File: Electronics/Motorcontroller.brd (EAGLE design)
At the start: 100 x 48.2 mm, 27 parts, among them Q1 IRFZ48V, Q2 IRF4905V, Q3 IRFZ48V, Q4 IRF4905V, Q5 IRFZ48V, Q6 IRF4905V, Q7 IRFZ48V, Q8 IRF4905V, X3 24V Batt

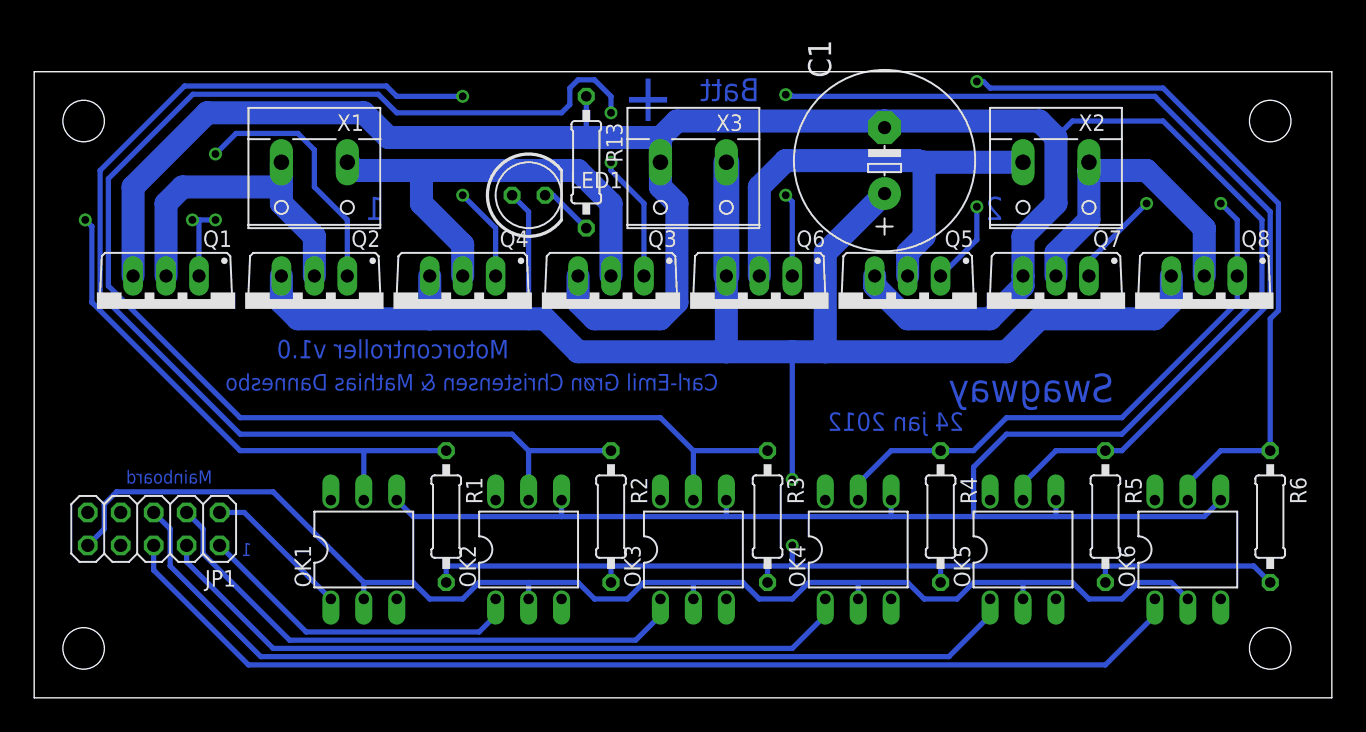
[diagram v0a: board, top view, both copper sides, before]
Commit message: Motorboard v2.0
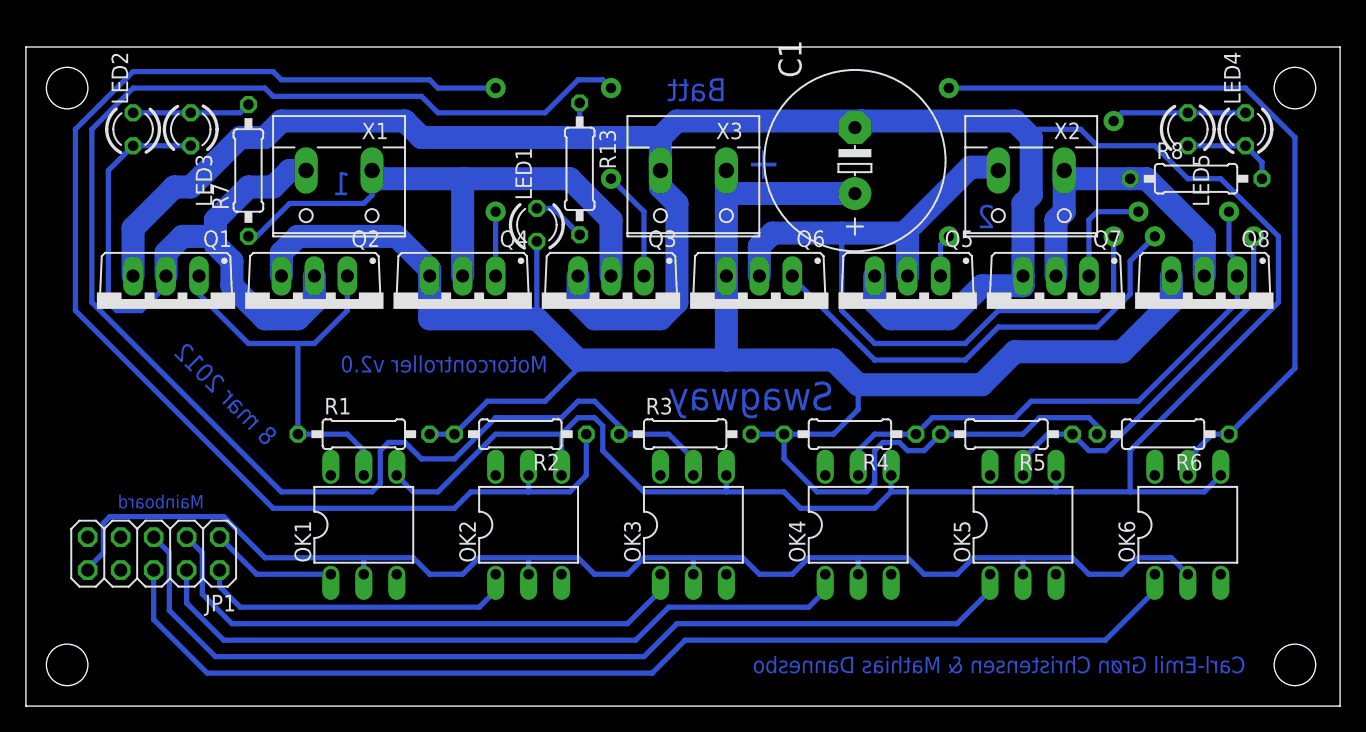
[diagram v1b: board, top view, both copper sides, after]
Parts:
- added LED2, LED3, LED4, LED5: (no value), led:LED3MM
- added R7, R8: 2.2k, rcl:0207/10
- LED1: device led:LED5MM -> led:LED3MM
- moved R6 10.4 mm to (87.0, 52.1), turned to 180 degrees
- moved R5 9.92 mm to (74.9, 52.1), turned to 180 degrees
- moved R2 9.44 mm to (37.5, 52.1), turned to 180 degrees
- moved R4 9.44 mm to (62.9, 52.1), turned to 180 degrees
- moved R1 8.98 mm to (25.4, 52.1), turned to 0 degrees
- moved R3 8.98 mm to (50.2, 52.1), turned to 0 degrees
- moved LED1 2.37 mm to (38.7, 68.2), turned to 90 degrees
- moved C1 2.29 mm to (63.2, 73.2)
- moved X1 2.01 mm to (23.5, 71.8)
- moved X2 2.01 mm to (76.8, 71.8)
- moved JP1 1.91 mm to (9.21, 42.9)
- moved OK1 1.91 mm to (25.4, 45.1)
- moved OK2 1.91 mm to (38.1, 45.1)
- moved OK3 1.91 mm to (50.8, 45.1)
- moved OK4 1.91 mm to (63.5, 45.1)
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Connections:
- removed net N$1: Q5.D, Q6.D, X2.2
- new net N$23: LED2.K, LED3.A, R7.2
- new net N$24: LED4.A, LED5.K, R8.2
- new net N$25: LED4.K, LED5.A, Q5.D, Q6.D, X2.2
- net N$18: now also R8.1
- net N$2: now also R7.1
- net N$4: now also LED2.A, LED3.K
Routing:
- net N$25: track 0.00 -> 71.1 mm, vias 0 -> 2
- net N$1: track 37.4 -> 0.00 mm
- net N$12: track 68.1 -> 32.6 mm, vias 2 -> 0
- net +24V: track 199.7 -> 170.5 mm, vias 2 -> 0
- net N$4: track 24.8 -> 53.8 mm
- net N$21: track 80.6 -> 66.3 mm, vias 1 -> 2
- net N$9: track 95.9 -> 106.1 mm
- net N$23: track 0.00 -> 9.15 mm
- net N$2: track 36.7 -> 44.5 mm
- net N$24: track 0.00 -> 7.51 mm
- net GND2: track 263.7 -> 258.9 mm
- net N$13: track 123.6 -> 126.6 mm, vias 1 -> 2
- net N$11: track 84.9 -> 86.6 mm
- net N$3: track 11.3 -> 9.76 mm
- net GND: track 102.6 -> 101.3 mm
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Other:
- board size 100 x 48.2 mm -> 101.3 x 50.8 mm
- board text added: "8 mar 2012"
- board text added: "Motorcontroller v2.0"
- board text removed: "24 jan 2012"
- board text removed: "Motorcontroller v1.0"
